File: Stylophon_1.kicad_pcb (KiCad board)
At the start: 2 copper layers, 57 x 38.5 mm, 75 parts, among them J4 Stylus, SW1 On/Off, SW2 Vibrato, T1 BC846, T2 BC846, U1 NE555D

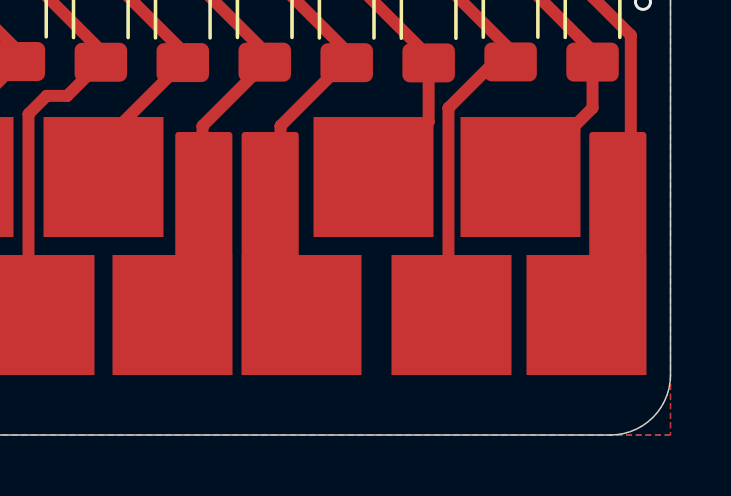
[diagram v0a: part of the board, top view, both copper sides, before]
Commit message: title
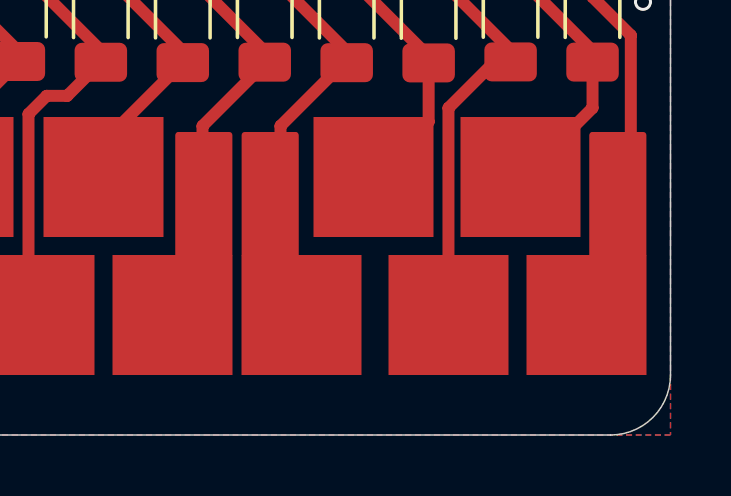
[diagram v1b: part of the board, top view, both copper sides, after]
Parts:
- moved TP3 0.10 mm to (163.0, 109.0)
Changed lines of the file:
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@@
 	)
 	(paper "A4")
+	(title_block
+		(title "Stylophone")
+		(rev "1.0")
+		(company "HTL Steyr")
+		(comment 1 "Gerrit Mitterhuemer")
+	)
 	(layers
 		(0 "F.Cu" signal)
@@
 	(footprint "Keypads:Keypad_Small"
 		(layer "F.Cu")
-		(at 163.1 109)
+		(at 163 109)
 		(descr "SMD rectangular pad as test Point, square 4.0mm side length")
 		(tags "test point SMD pad rectangle square")
